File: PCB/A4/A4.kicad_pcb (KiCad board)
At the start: 2 copper layers, 88.3 x 68.3 mm, 78 parts, among them J1 Barrel_Jack_Switch, J10 Conn_02x03_Odd_Even, J11 Conn_01x04_Male, J12 Conn_01x04_Male, J13 Conn_01x06_Male, J14 Conn_01x02_Male, J15 Conn_01x06_Male, J16 Conn_01x02_Male, J17 Conn_01x06_Male, J18 Conn_01x06_Male, J19 Conn_02x03_Odd_Even, J2 Conn_01x02_Male, J20 Conn_02x03_Odd_Even, J21 Conn_01x04_Male, J22 Conn_01x04_Male, J23 Conn_01x02_Male, J24 Conn_01x02_Male, J3 Conn_01x06_Male, J4 Conn_01x02_Male, J5 Conn_01x06_Male, J6 Conn_01x06_Male, J7 Screw_Terminal_01x02, J8 Screw_Terminal_01x02, J9 Conn_02x03_Odd_Even, Q1 2N7002, Q10 2N7002, Q11 2N7002, Q12 2N7002, Q2 2N7002, Q3 2N7002, Q4 2N7002, Q5 2N7002, Q6 2N7002, Q7 2N7002, Q8 2N7002, Q9 2N7002, U1 AZ1117-3.3, U2 TB67H451FNG,EL, U3 ESP32-S2-WROOM, U4 TB67H451FNG,EL, U5 AZ1117-5.0

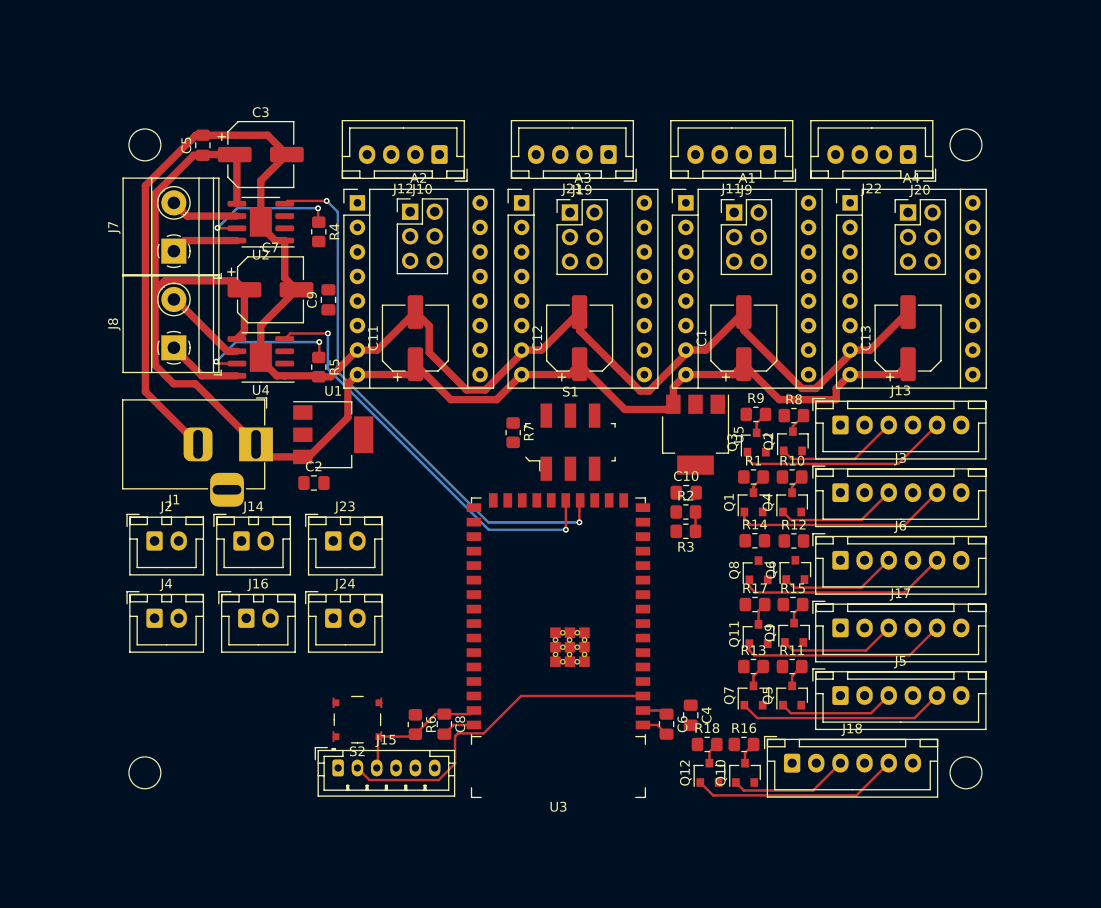
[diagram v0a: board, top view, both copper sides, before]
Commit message: PCB ready to order
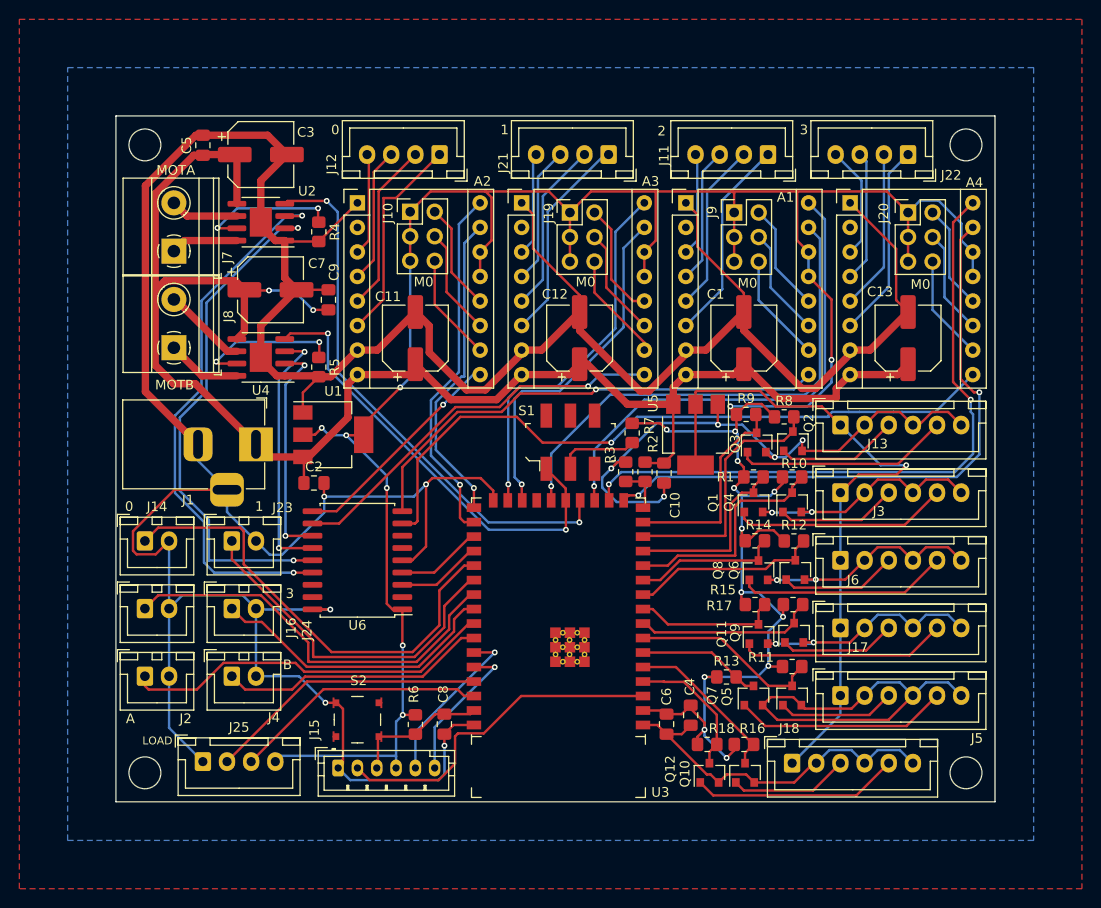
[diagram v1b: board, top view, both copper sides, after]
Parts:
- added J25: Conn_01x04_Male, Connector_JST:JST_XH_B4B-XH-A_1x04_P2.50mm_Vertical, F.Cu at (174.0, 116.8)
- added U6: MCP23009, Package_SO:SOIC-18W_7.5x11.6mm_P1.27mm, F.Cu at (190.0, 96.0)
- moved J2 14.0 mm to (168.0, 108.0)
- moved R7 12.3 mm to (218.4, 82.8)
- moved J16 10.5 mm to (168.0, 101.0)
- moved J24 10.5 mm to (177.0, 101.0)
- moved J23 10.5 mm to (177.0, 94.0)
- moved J14 10.0 mm to (168.0, 94.0)
- moved J4 10.0 mm to (177.0, 108.0)
- moved R3 8.76 mm to (217.8, 86.8), turned to 90 degrees
- moved R2 5.93 mm to (219.8, 86.8), turned to 270 degrees
- moved C10 3.06 mm to (221.7, 87.0), turned to 270 degrees
- moved R13 3.00 mm to (228.2, 108.1)
- moved R8 1.02 mm to (234.2, 81.2)
- moved R9 1.02 mm to (230.2, 80.9)
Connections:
- Q9 pad 3: ENC1 -> ENC1A
- R15 pad 2: ENC1 -> ENC1A
- U3 pad 10: ENCBA -> ENC0A
- U3 pad 11: ENCBB -> ENC0B
- U3 pad 12: CHARGE -> ENCBA
- U3 pad 13: DIR0 -> ENCBB
- U3 pad 14: STEP0 -> ENCAA
- U3 pad 15: EN0 -> ENCAB
- U3 pad 16: DIR1 -> CHARGE
- U3 pad 17: STEP1 -> STEP3
- U3 pad 18: EN1 -> DIR3
- U3 pad 23: EN2 -> Net-(U3-Pad23)
- U3 pad 24: DIR3 -> STEP1
- U3 pad 25: STEP3 -> DIR1
- U3 pad 27: EN3 -> STEP0
- U3 pad 28: HOM0 -> DIR0
- U3 pad 29: HOM1 -> SDA
- U3 pad 30: HOM2 -> SCL
- U3 pad 31: HOM3 -> HOM0
- U3 pad 32: HOMA -> HOM1
- U3 pad 33: HOMB -> HOM2
- U3 pad 34: Net-(U3-Pad34) -> HOM3
- U3 pad 35: Net-(U3-Pad35) -> HOMA
- U3 pad 36: Net-(U3-Pad36) -> HOMB
- U3 pad 39: Net-(U3-Pad39) -> DAT
- U3 pad 4: MOTA1 -> ENC3B
- U3 pad 40: Net-(U3-Pad40) -> CLK
- U3 pad 5: MOTA2 -> ENC3A
- U3 pad 6: ENCAA -> ENC2B
- U3 pad 7: ENCAB -> ENC2A
- U3 pad 8: MOTB1 -> ENC1A
- U3 pad 9: MOTB2 -> ENC1B
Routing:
- net GND: track 174.4 -> 598.4 mm, vias 0 -> 16
- net +3V3: track 2.60 -> 314.6 mm, vias 0 -> 20
- net EN3: track 0.00 -> 71.5 mm, vias 0 -> 1
- net +5V: track 0.00 -> 70.7 mm, vias 0 -> 1
- net DIR3: track 0.00 -> 68.4 mm, vias 0 -> 2
- net STEP3: track 0.00 -> 64.0 mm, vias 0 -> 2
- net MOTA1: track 0.00 -> 57.0 mm, vias 0 -> 2
- net MOTA2: track 0.00 -> 53.9 mm, vias 0 -> 2
- net STEP2: track 0.00 -> 52.1 mm, vias 0 -> 1
- net DIR2: track 0.00 -> 51.3 mm, vias 0 -> 1
- net EN2: track 0.00 -> 50.6 mm, vias 0 -> 1
- net HOM0: track 0.00 -> 47.8 mm
- net HOM2: track 0.00 -> 42.4 mm
- net EN1: track 0.00 -> 40.7 mm, vias 0 -> 1
- net DIR1: track 0.00 -> 38.9 mm, vias 0 -> 1
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- added copper zone on F.Cu, net +3V3
- added copper zone on B.Cu, net GND
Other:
- board size 88.3 x 68.3 mm -> 91 x 71 mm
- board text added: "0"
- board text added: "1"
- board text added: "2"
- board text added: "3"
- board text added: "A"
- board text added: "B"
- board text added: "ENC0"
- board text added: "ENC1"
- board text added: "ENC2"
- board text added: "ENC3"
- board text added: "ENCA"
- board text added: "ENCB"
- board text added: "LOAD"
- board text added: "M0"
- board text added: "MOTA"
- board text added: "MOTB"
- board text added: "PROGRAM"
- board text added: "SAGE ROBOTS A4 2.0"
